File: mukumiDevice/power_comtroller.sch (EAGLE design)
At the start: 46 parts, among them IC5 ATMEGA328-20P

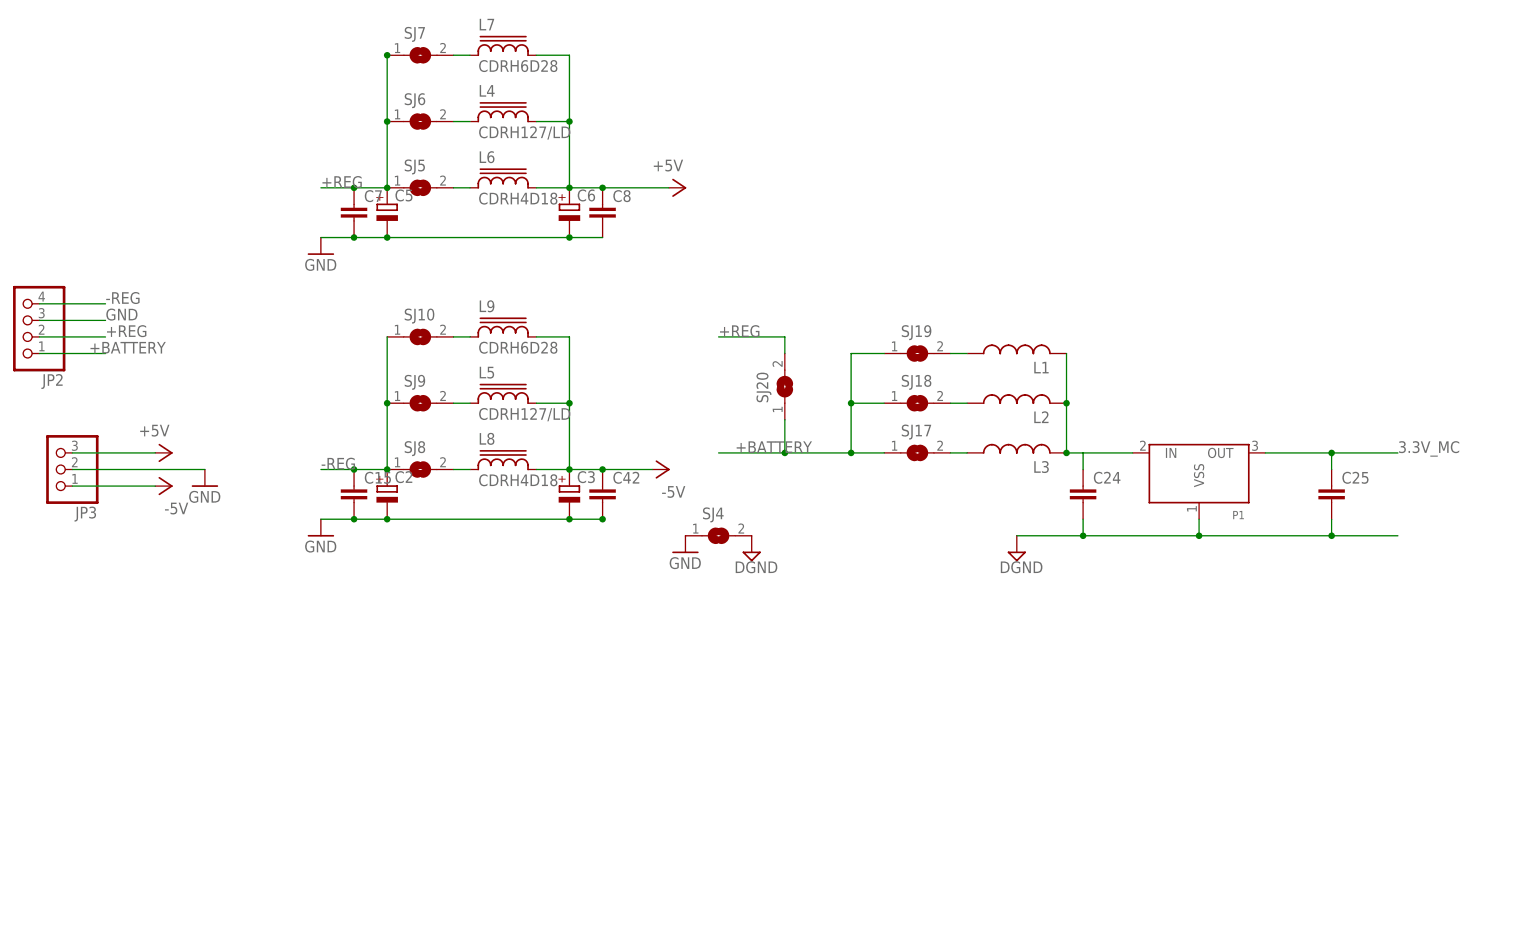
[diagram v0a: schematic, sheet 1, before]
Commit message: addAnalogPowerFilter
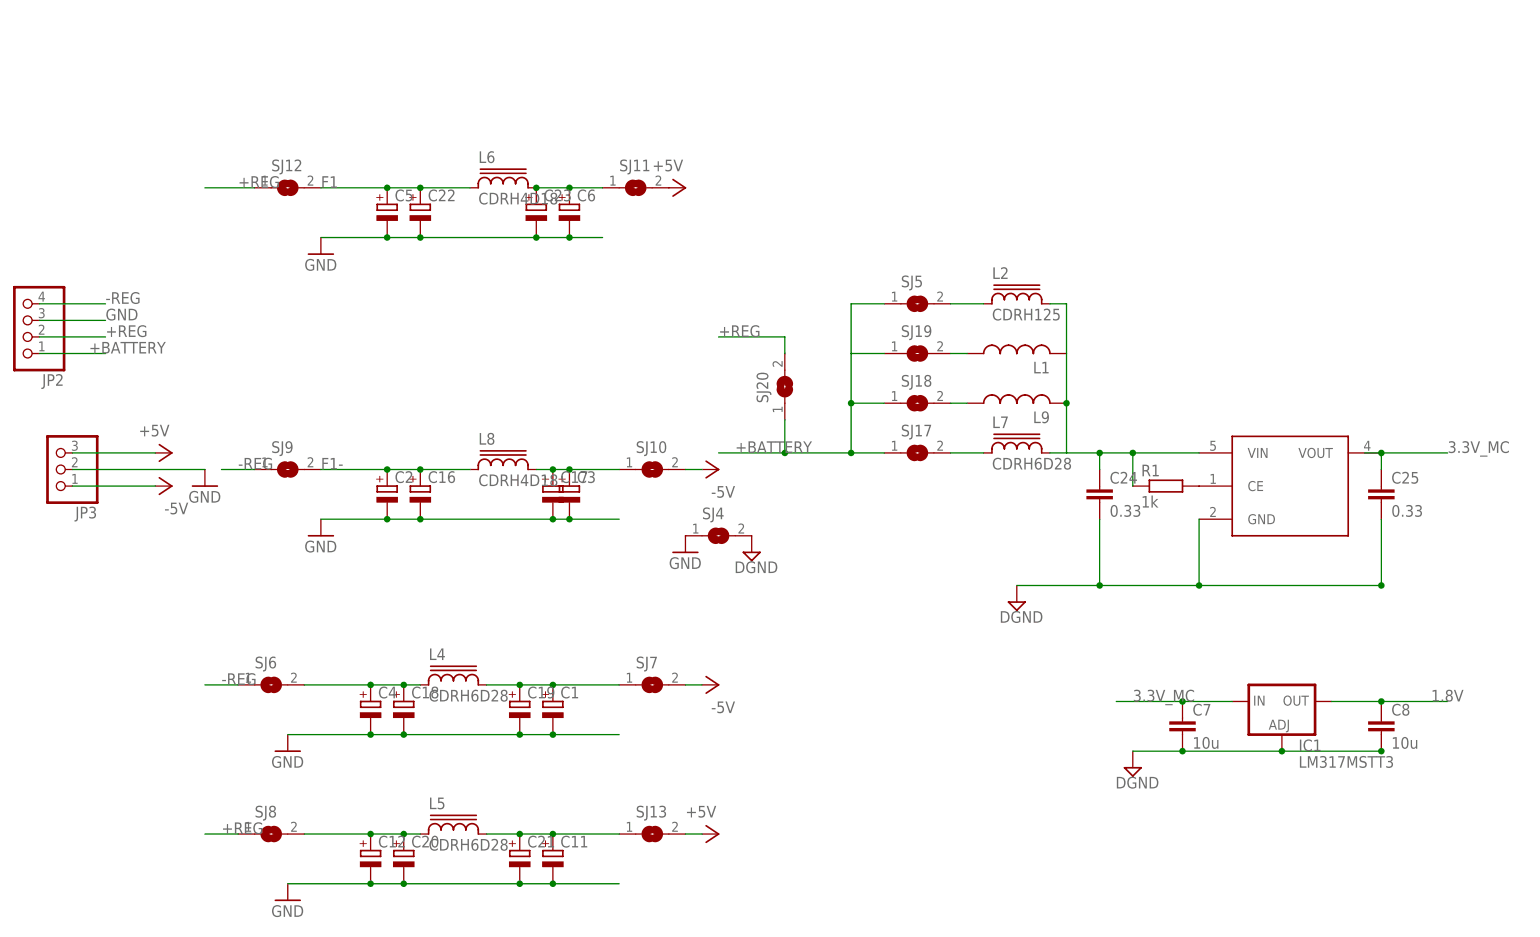
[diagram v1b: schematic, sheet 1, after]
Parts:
- removed C15, C42: (no value), rcl:C-EUC0805
- removed L3: (no value), rcl:L-USL2825P
- removed P1: (no value), Voltage Regulator:XC6206SOT-89
- added C1, C11, C12, C4: (no value), rcl:CPOL-EUTT2D6
- added C16, C17, C18, C19, C20, C21, C22, C23: (no value), rcl:CPOL-EUD/7343-31W
- added IC1: LM317MSTT3, v-reg:LM317MSTT3
- added R1: 1k, rcl:R-EU_0204/2V
- added SJ11, SJ12, SJ13: (no value), jumper:SJ
- added U$1: NJM2884, torex:NJM2884
- C24, C25: value (none) -> 0.33
- C7, C8: value (none) -> 10u; device rcl:C-EU025-030X050 -> rcl:C-EUC0402
- L2: value (none) -> CDRH125; device rcl:L-USL3225P -> inductor-sumida:CDRH125
- L4, L5: value CDRH127/LD -> CDRH6D28; device inductor-sumida:CDRH127/LD -> inductor-sumida:CDRH6D28
- L9: value CDRH6D28 -> (none); device inductor-sumida:CDRH6D28 -> rcl:L-USL2825P
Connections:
- removed net N$17: L8.1, SJ8.2
- removed net N$6: L5.1, SJ9.2
- new net 1.8V: C8.1, IC1.OUT
- new net F1: C22.+, C5.+, L6.1, SJ12.2
- new net F1-: C16.+, C2.+, L8.1, SJ9.2
- new net F2: C12.+, C20.+, L5.1, SJ8.2
- new net F2-: C18.+, C4.+, L4.1, SJ6.2
- new net N$1: C23.+, C6.+, L6.2, SJ11.1
- new net N$7: C11.+, C21.+, L5.2, SJ13.1
- net +5V: now also SJ11.2, SJ13.2; no longer C6.+, C8.1, L4.2, L6.2, L7.2
- net +BATTERY: now also SJ5.1
- net +REG: now also SJ12.1, SJ8.1; no longer C5.+, C7.1, SJ5.1, SJ6.1, SJ7.1
- net -5V: now also SJ10.2, SJ7.2; no longer C3.+, C42.1, L5.2, L8.2, L9.2
- net -REG: now also SJ6.1; no longer C15.1, C2.+, SJ10.1, SJ8.1
- net 3.3V_MC: now also C7.1, IC1.IN, U$1.VOUT; no longer P1.OUT
- net DGND: now also C7.2, C8.2, IC1.ADJ, U$1.GND; no longer P1.VSS
- net GND: now also C1.-, C11.-, C12.-, C16.-, C17.-, C18.-, C19.-, C20.-, C21.-, C22.-, C23.-, C4.-; no longer C15.2, C42.2, C7.2, C8.2
- net N$19: now also L7.2, L9.2, R1.1, U$1.VIN; no longer L3.2, P1.IN
- net N$2: now also R1.2, U$1.CE; no longer L7.1, SJ7.2
- net N$29: now also L7.1; no longer L3.1
- net N$3: now also C1.+, C19.+, L4.2, SJ7.1; no longer L4.1, SJ6.2
- net N$38: now also L9.1; no longer L2.1
- net N$4: now also L2.1; no longer L6.1
- net N$5: now also C17.+, C3.+, L8.2, SJ10.1; no longer L9.1, SJ10.2
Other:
- moved on the sheet: C24, C25, C7, C8, L2, L4, L5, L7, L9, SJ10, SJ5, SJ6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
